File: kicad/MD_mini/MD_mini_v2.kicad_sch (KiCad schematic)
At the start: 82 parts, among them J1 Conn_01x02_Pin, J2 Conn_01x04_Pin, J3 Conn_01x02_Pin, J4 Conn_01x02_Pin, J6 Conn_02x03_Odd_Even, U1 IRS2003, U2 SCM3723ASA, U3 IRS2003, U4 ACS711xEXLT-15AB, U6 ACS711xEXLT-15AB, U7 IRS2003, U8 IRS2003, U9 SCM3723ASA

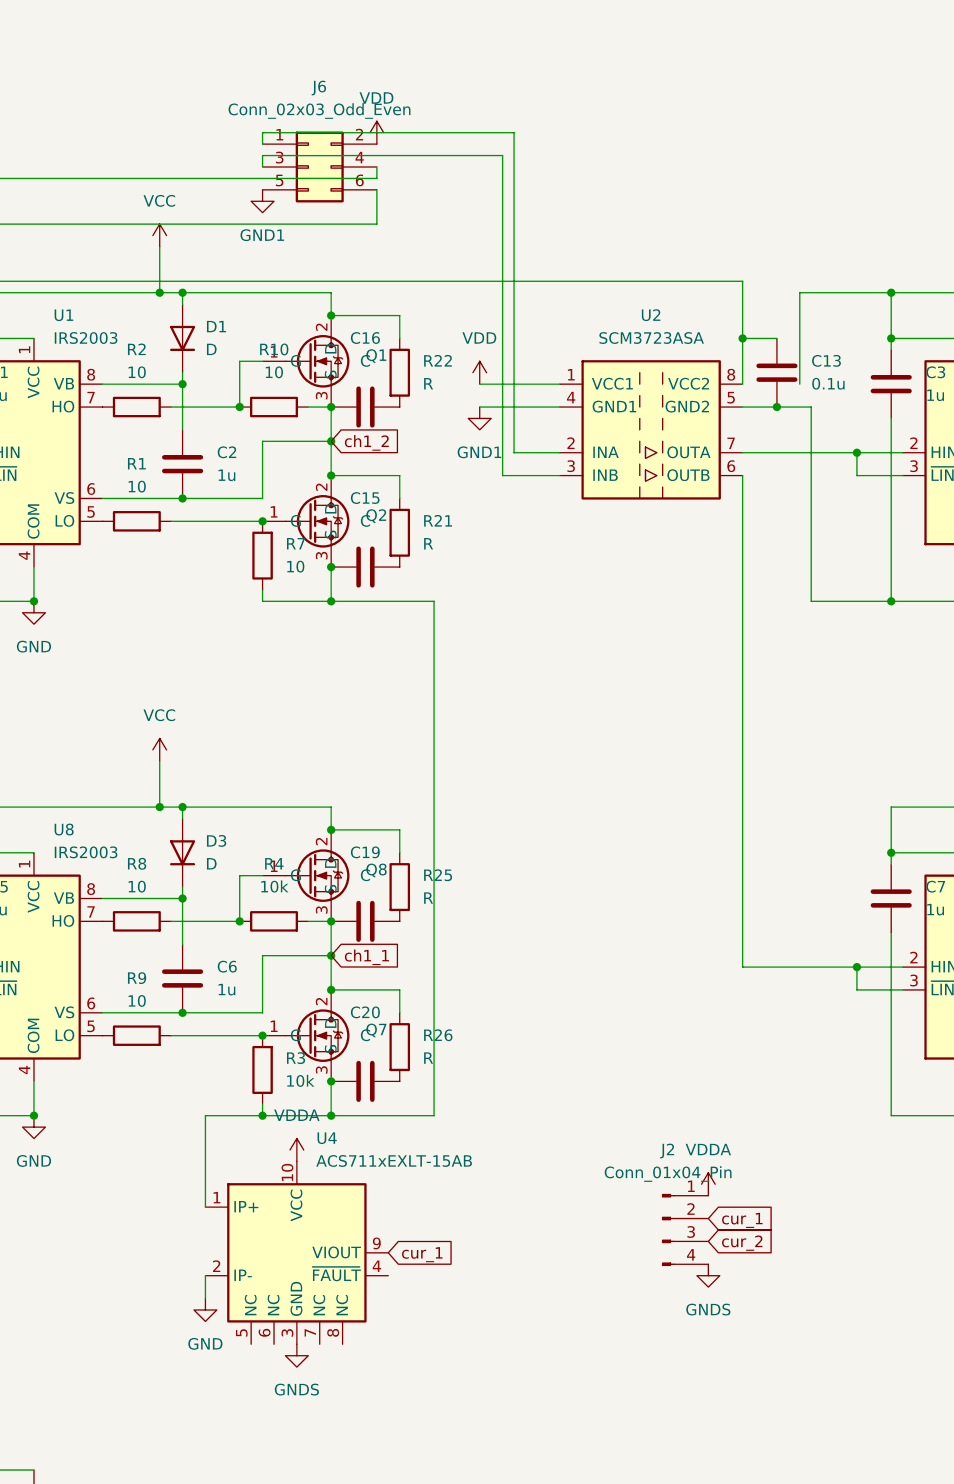
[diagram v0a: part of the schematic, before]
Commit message: a
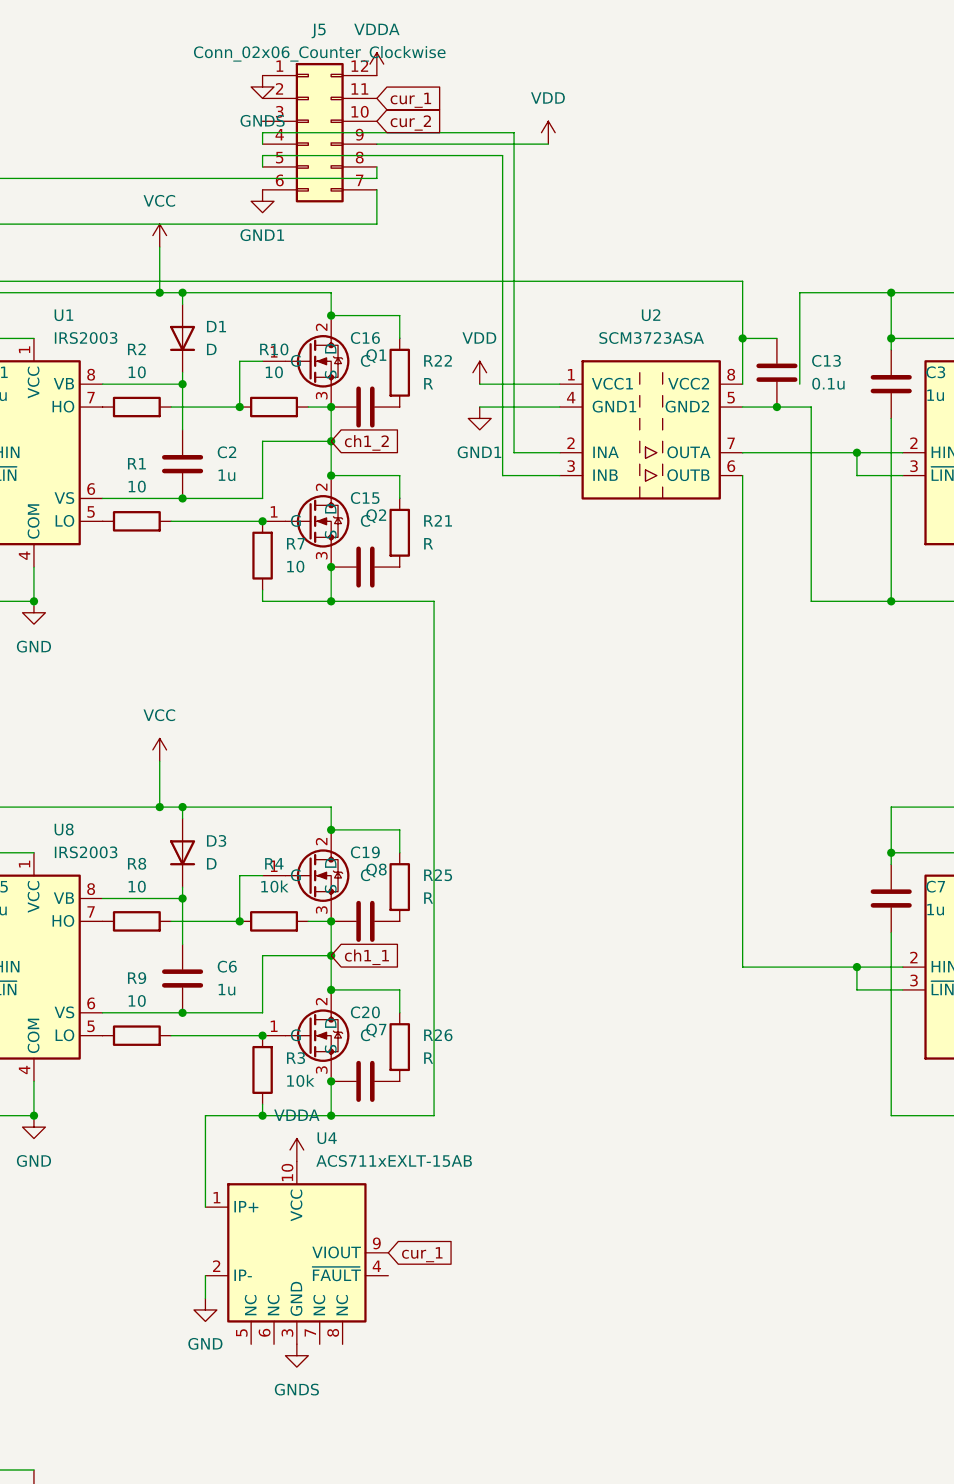
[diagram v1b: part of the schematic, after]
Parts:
- removed J2: Conn_01x04_Pin, Connector_PinHeader_2.54mm:PinHeader_1x04_P2.54mm_Vertical, symbol Connector:Conn_01x04_Pin
- removed J6: Conn_02x03_Odd_Even, Connector_PinHeader_2.54mm:PinHeader_2x03_P2.54mm_Horizontal, symbol Connector_Generic:Conn_02x03_Odd_Even
- added J5: Conn_02x06_Counter_Clockwise, symbol Connector_Generic:Conn_02x06_Counter_Clockwise
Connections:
- net GND1: now also J5.6 (Pin_6)
- net GNDS: now also J5.1 (Pin_1)
- net VDD: now also J5.9 (Pin_9)
- net VDDA: now also J5.12 (Pin_12)
- net cur_1: now also J5.11 (Pin_11)
- net cur_2: now also J5.10 (Pin_10)
- net at U9.2 (INA): now also J5.7 (Pin_7)
- net at U9.3 (INB): now also J5.8 (Pin_8)
- net at U2.2 (INA): now also J5.4 (Pin_4)
- net at U2.3 (INB): now also J5.5 (Pin_5)
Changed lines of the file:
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@@
 	(wire
 		(pts
+			(xy 156.21 15.24) (xy 137.16 15.24)
+		)
+		(stroke
+			(width 0)
+			(type default)
+		)
+	)
+	(wire
+		(pts
 			(xy 124.46 13.97) (xy 152.4 13.97)
 		)
@@
 		)
 	)
-	(global_label "cur_1"
+	(global_label "ch2_1"
 		(shape input)
-		(at 173.99 134.62 0)
+		(at 236.22 105.41 0)
 		(fields_autoplaced yes)
 		(effects
@@
 		)
 		(property "Intersheetrefs" "${INTERSHEET_REFS}"
-			(at 182.1761 134.62 0)
+			(at 244.8294 105.41 0)
 			(effects
 				(font
@@
 	(global_label "ch2_1"
 		(shape input)
-		(at 236.22 105.41 0)
+		(at 25.4 121.92 0)
 		(fields_autoplaced yes)
 		(effects
@@
 		)
 		(property "Intersheetrefs" "${INTERSHEET_REFS}"
-			(at 244.8294 105.41 0)
+			(at 34.0094 121.92 0)
 			(effects
 				(font
@@
 		)
 	)
-	(global_label "ch2_1"
+	(global_label "cur_1"
 		(shape input)
-		(at 25.4 121.92 0)
+		(at 137.16 10.16 0)
 		(fields_autoplaced yes)
 		(effects
@@
 		)
 		(property "Intersheetrefs" "${INTERSHEET_REFS}"
-			(at 34.0094 121.92 0)
+			(at 145.3461 10.16 0)
 			(effects
 				(font
@@
 	(global_label "cur_2"
 		(shape input)
-		(at 173.99 137.16 0)
+		(at 137.16 12.7 0)
 		(fields_autoplaced yes)
 		(effects
@@
 		)
 		(property "Intersheetrefs" "${INTERSHEET_REFS}"
-			(at 182.1761 137.16 0)
+			(at 145.3461 12.7 0)
 			(effects
 				(font
@@
 	)
 	(symbol
-		(lib_id "Connector:Conn_01x04_Pin")
-		(at 168.91 134.62 0)
-		(unit 1)
-		(exclude_from_sim no)
-		(in_bom yes)
-		(on_board yes)
-		(dnp no)
-		(fields_autoplaced yes)
-		(property "Reference" "J2"
-			(at 169.545 127 0)
-			(effects
-				(font
-					(size 1.27 1.27)
-				)
-			)
-		)
-		(property "Value" "Conn_01x04_Pin"
-			(at 169.545 129.54 0)
-			(effects
-				(font
-					(size 1.27 1.27)
-				)
-			)
-		)
-		(property "Footprint" "Connector_PinHeader_2.54mm:PinHeader_1x04_P2.54mm_Vertical"
-			(at 168.91 134.62 0)
-			(effects
-				(font
-					(size 1.27 1.27)
-				)
-				(hide yes)
-			)
-		)
-		(property "Datasheet" "~"
-			(at 168.91 134.62 0)
-			(effects
-				(font
-					(size 1.27 1.27)
-				)
-				(hide yes)
-			)
-		)
-		(property "Description" "Generic connector, single row, 01x04, script generated"
-			(at 168.91 134.62 0)
-			(effects
-				(font
-					(size 1.27 1.27)
-				)
-				(hide yes)
-			)
-		)
-		(pin "3"
-		)
-		(pin "2"
-		)
-		(pin "4"
-		)
-		(pin "1"
-		)
-		(instances
-			(project ""
-				(path "/5b9174b4-8dcf-442c-9b99-056da30be3d5"
-					(reference "J2")
-					(unit 1)
-				)
-			)
-		)
-	)
-	(symbol
 		(lib_id "Device:C")
 		(at 240.03 119.38 90)
@@
 	(symbol
 		(lib_id "power:VDDA")
-		(at 173.99 132.08 0)
+		(at 137.16 7.62 0)
 		(unit 1)
 		(exclude_from_sim no)
@@
 		(fields_autoplaced yes)
 		(property "Reference" "#PWR021"
-			(at 173.99 135.89 0)
+			(at 137.16 11.43 0)
 			(effects
 				(font
@@
 		)
 		(property "Value" "VDDA"
-			(at 173.99 127 0)
+			(at 137.16 2.54 0)
 			(effects
 				(font
@@
 		)
 		(property "Footprint" ""
-			(at 173.99 132.08 0)
+			(at 137.16 7.62 0)
 			(effects
 				(font
@@
 		)
 		(property "Datasheet" ""
-			(at 173.99 132.08 0)
+			(at 137.16 7.62 0)
 			(effects
 				(font
@@
 		)
 		(property "Description" "Power symbol creates a global label with name \"VDDA\""
-			(at 173.99 132.08 0)
+			(at 137.16 7.62 0)
 			(effects
 				(font
@@
 		)
 		(instances
-			(project "MD_mini"
+			(project "MD_mini_v2"
 				(path "/5b9174b4-8dcf-442c-9b99-056da30be3d5"
 					(reference "#PWR021")
@@
 	)
 	(symbol
+		(lib_id "Connector_Generic:Conn_02x06_Counter_Clockwise")
+		(at 129.54 12.7 0)
+		(unit 1)
+		(exclude_from_sim no)
+		(in_bom yes)
+		(on_board yes)
+		(dnp no)
+		(fields_autoplaced yes)
+		(property "Reference" "J5"
+			(at 130.81 2.54 0)
+			(effects
+				(font
+					(size 1.27 1.27)
+				)
+			)
+		)
+		(property "Value" "Conn_02x06_Counter_Clockwise"
+			(at 130.81 5.08 0)
+			(effects
+				(font
+					(size 1.27 1.27)
+				)
+			)
+		)
+		(property "Footprint" ""
+			(at 129.54 12.7 0)
+			(effects
+				(font
+					(size 1.27 1.27)
+				)
+				(hide yes)
+			)
+		)
+		(property "Datasheet" "~"
+			(at 129.54 12.7 0)
+			(effects
+				(font
+					(size 1.27 1.27)
+				)
+				(hide yes)
+			)
+		)
+		(property "Description" "Generic connector, double row, 02x06, counter clockwise pin numbering scheme (similar to DIP package numbering), script generated (kicad-library-utils/schlib/autogen/connector/)"
+			(at 129.54 12.7 0)
+			(effects
+				(font
+					(size 1.27 1.27)
+				)
+				(hide yes)
+			)
+		)
+		(pin "11"
+		)
+		(pin "2"
+		)
+		(pin "12"
+		)
+		(pin "7"
+		)
+		(pin "6"
+		)
+		(pin "8"
+		)
+		(pin "9"
+		)
+		(pin "5"
+		)
+		(pin "10"
+		)
+		(pin "1"
+		)
+		(pin "3"
+		)
+		(pin "4"
+		)
+		(instances
+			(project ""
+				(path "/5b9174b4-8dcf-442c-9b99-056da30be3d5"
+					(reference "J5")
+					(unit 1)
+				)
+			)
+		)
+	)
+	(symbol
 		(lib_id "Device:R")
 		(at 139.7 40.64 0)
@@
 	)
 	(symbol
-		(lib_id "Connector_Generic:Conn_02x03_Odd_Even")
-		(at 129.54 17.78 0)
-		(unit 1)
-		(exclude_from_sim no)
-		(in_bom yes)
-		(on_board yes)
-		(dnp no)
-		(fields_autoplaced yes)
-		(property "Reference" "J6"
-			(at 130.81 8.89 0)
-			(effects
-				(font
-					(size 1.27 1.27)
-				)
-			)
-		)
-		(property "Value" "Conn_02x03_Odd_Even"
-			(at 130.81 11.43 0)
-			(effects
-				(font
-					(size 1.27 1.27)
-				)
-			)
-		)
-		(property "Footprint" "Connector_PinHeader_2.54mm:PinHeader_2x03_P2.54mm_Horizontal"
-			(at 129.54 17.78 0)
-			(effects
-				(font
-					(size 1.27 1.27)
-				)
-				(hide yes)
-			)
-		)
-		(property "Datasheet" "~"
-			(at 129.54 17.78 0)
-			(effects
-				(font
-					(size 1.27 1.27)
-				)
-				(hide yes)
-			)
-		)
-		(property "Description" "Generic connector, double row, 02x03, odd/even pin numbering scheme (row 1 odd numbers, row 2 even numbers), script generated (kicad-library-utils/schlib/autogen/connector/)"
-			(at 129.54 17.78 0)
-			(effects
-				(font
-					(size 1.27 1.27)
-				)
-				(hide yes)
-			)
-		)
-		(pin "2"
-		)
-		(pin "1"
-		)
-		(pin "5"
-		)
-		(pin "4"
-		)
-		(pin "6"
-		)
-		(pin "3"
-		)
-		(instances
-			(project ""
-				(path "/5b9174b4-8dcf-442c-9b99-056da30be3d5"
-					(reference "J6")
-					(unit 1)
-				)
-			)
-		)
-	)
-	(symbol
 		(lib_id "jisaku:RD3L07BBG")
 		(at 234.95 57.15 0)
@@
 	(symbol
 		(lib_id "power:VDD")
-		(at 137.16 15.24 0)
+		(at 156.21 15.24 0)
 		(unit 1)
 		(exclude_from_sim no)
@@
 		(fields_autoplaced yes)
 		(property "Reference" "#PWR03"
-			(at 137.16 19.05 0)
+			(at 156.21 19.05 0)
 			(effects
 				(font
@@
 		)
 		(property "Value" "VDD"
-			(at 137.16 10.16 0)
+			(at 156.21 10.16 0)
 			(effects
 				(font
@@
 		)
 		(property "Footprint" ""
-			(at 137.16 15.24 0)
+			(at 156.21 15.24 0)
 			(effects
 				(font
@@
 		)
 		(property "Datasheet" ""
-			(at 137.16 15.24 0)
+			(at 156.21 15.24 0)
 			(effects
 				(font
@@
 		)
 		(property "Description" "Power symbol creates a global label with name \"VDD\""
-			(at 137.16 15.24 0)
+			(at 156.21 15.24 0)
 			(effects
 				(font
@@
 	(symbol
 		(lib_id "power:GNDS")
-		(at 173.99 139.7 0)
+		(at 124.46 7.62 0)
 		(unit 1)
 		(exclude_from_sim no)
@@
 		(fields_autoplaced yes)
 		(property "Reference" "#PWR020"
-			(at 173.99 146.05 0)
+			(at 124.46 13.97 0)
 			(effects
 				(font
@@
 		)
 		(property "Value" "GNDS"
-			(at 173.99 144.78 0)
+			(at 124.46 12.7 0)
 			(effects
 				(font
@@
 		)
 		(property "Footprint" ""
-			(at 173.99 139.7 0)
+			(at 124.46 7.62 0)
 			(effects
 				(font
@@
 		)
 		(property "Datasheet" ""
-			(at 173.99 139.7 0)
+			(at 124.46 7.62 0)
 			(effects
 				(font
@@
 		)
 		(property "Description" "Power symbol creates a global label with name \"GNDS\" , signal ground"
-			(at 173.99 139.7 0)
+			(at 124.46 7.62 0)
 			(effects
 				(font
@@
 		)
 		(instances
-			(project "MD_mini"
+			(project "MD_mini_v2"
 				(path "/5b9174b4-8dcf-442c-9b99-056da30be3d5"
 					(reference "#PWR020")

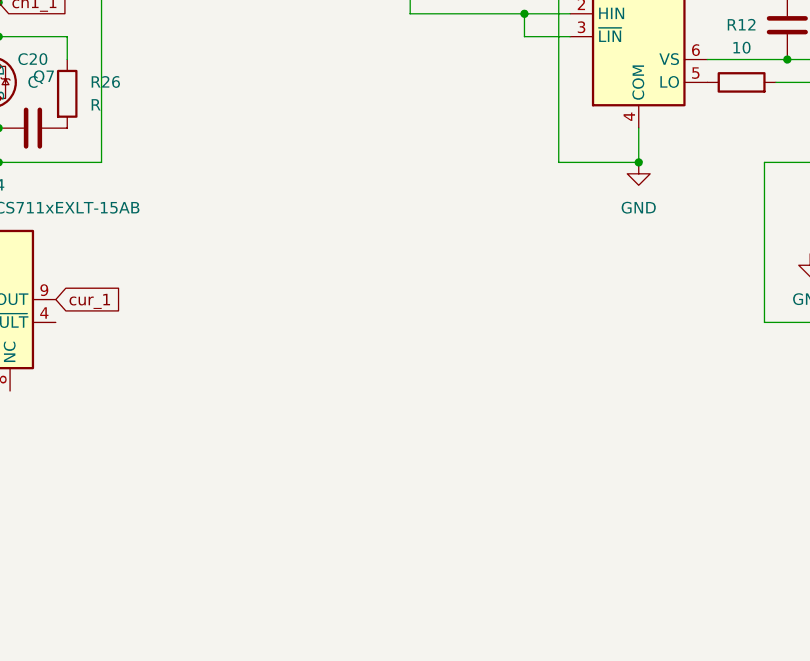
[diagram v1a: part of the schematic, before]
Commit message: a
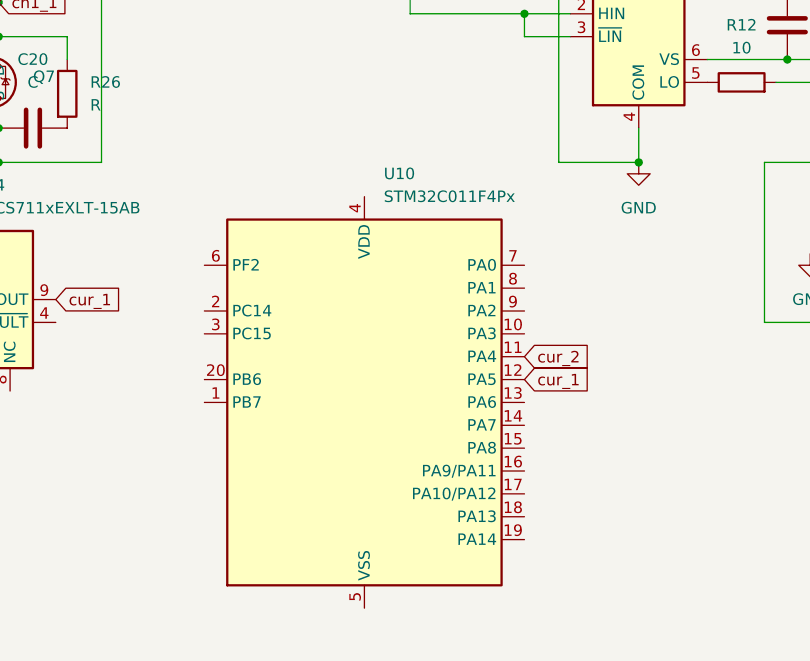
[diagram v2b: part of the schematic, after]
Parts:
- added U10: STM32C011F4Px, Package_SO:TSSOP-20_4.4x6.5mm_P0.65mm, symbol MCU_ST_STM32C0:STM32C011F4Px
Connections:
- net cur_1: now also U10.12 (PA5)
- net cur_2: now also U10.11 (PA4)
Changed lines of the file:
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@@
 		)
 	)
+	(global_label "cur_1"
+		(shape input)
+		(at 190.5 147.32 0)
+		(fields_autoplaced yes)
+		(effects
+			(font
+				(size 1.27 1.27)
+			)
+			(justify left)
+		)
+		(property "Intersheetrefs" "${INTERSHEET_REFS}"
+			(at 198.6861 147.32 0)
+			(effects
+				(font
+					(size 1.27 1.27)
+				)
+				(justify left)
+				(hide yes)
+			)
+		)
+	)
 	(global_label "cur_2"
 		(shape input)
@@
 		)
 	)
+	(global_label "cur_2"
+		(shape input)
+		(at 190.5 144.78 0)
+		(fields_autoplaced yes)
+		(effects
+			(font
+				(size 1.27 1.27)
+			)
+			(justify left)
+		)
+		(property "Intersheetrefs" "${INTERSHEET_REFS}"
+			(at 198.6861 144.78 0)
+			(effects
+				(font
+					(size 1.27 1.27)
+				)
+				(justify left)
+				(hide yes)
+			)
+		)
+	)
 	(global_label "ch2_1"
 		(shape input)
@@
 					(unit 1)
 				)
+			)
+		)
+	)
+	(symbol
+		(lib_id "MCU_ST_STM32C0:STM32C011F4Px")
+		(at 172.72 149.86 0)
+		(unit 1)
+		(exclude_from_sim no)
+		(in_bom yes)
+		(on_board yes)
+		(dnp no)
+		(fields_autoplaced yes)
+		(property "Reference" "U10"
+			(at 174.8633 124.46 0)
+			(effects
+				(font
+					(size 1.27 1.27)
+				)
+				(justify left)
+			)
+		)
+		(property "Value" "STM32C011F4Px"
+			(at 174.8633 127 0)
+			(effects
+				(font
+					(size 1.27 1.27)
+				)
+				(justify left)
+			)
+		)
+		(property "Footprint" "Package_SO:TSSOP-20_4.4x6.5mm_P0.65mm"
+			(at 157.48 170.18 0)
+			(effects
+				(font
+					(size 1.27 1.27)
+				)
+				(justify right)
+				(hide yes)
+			)
+		)
+		(property "Datasheet" "https://www.st.com/resource/en/datasheet/stm32c011f4.pdf"
+			(at 172.72 149.86 0)
+			(effects
+				(font
+					(size 1.27 1.27)
+				)
+				(hide yes)
+			)
+		)
+		(property "Description" "STMicroelectronics Arm Cortex-M0+ MCU, 16KB flash, 6KB RAM, 48 MHz, 2.0-3.6V, 18 GPIO, TSSOP20"
+			(at 172.72 149.86 0)
+			(effects
+				(font
+					(size 1.27 1.27)
+				)
+				(hide yes)
+			)
+		)
+		(pin "9"
+		)
+		(pin "2"
+		)
+		(pin "14"
+		)
+		(pin "20"
+		)
+		(pin "19"
+		)
+		(pin "7"
+		)
+		(pin "4"
+		)
+		(pin "6"
+		)
+		(pin "1"
+		)
+		(pin "5"
+		)
+		(pin "10"
+		)
+		(pin "3"
+		)
+		(pin "8"
+		)
+		(pin "12"
+		)
+		(pin "11"
+		)
+		(pin "15"
+		)
+		(pin "16"
+		)
+		(pin "13"
+		)
+		(pin "17"
+		)
+		(pin "18"
+		)
+		(instances
+			(project ""
+				(path "/5b9174b4-8dcf-442c-9b99-056da30be3d5"
+					(reference "U10")
+					(unit 1)
+				)
